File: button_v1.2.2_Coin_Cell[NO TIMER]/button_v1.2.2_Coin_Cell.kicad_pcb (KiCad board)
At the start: 2 copper layers, 21 x 47.8 mm, 18 parts, among them J1 Conn_01x05_Female, SW1 SW_Push, SW2 SW_Push, U1 TPS61097A, X1 ESP-12E

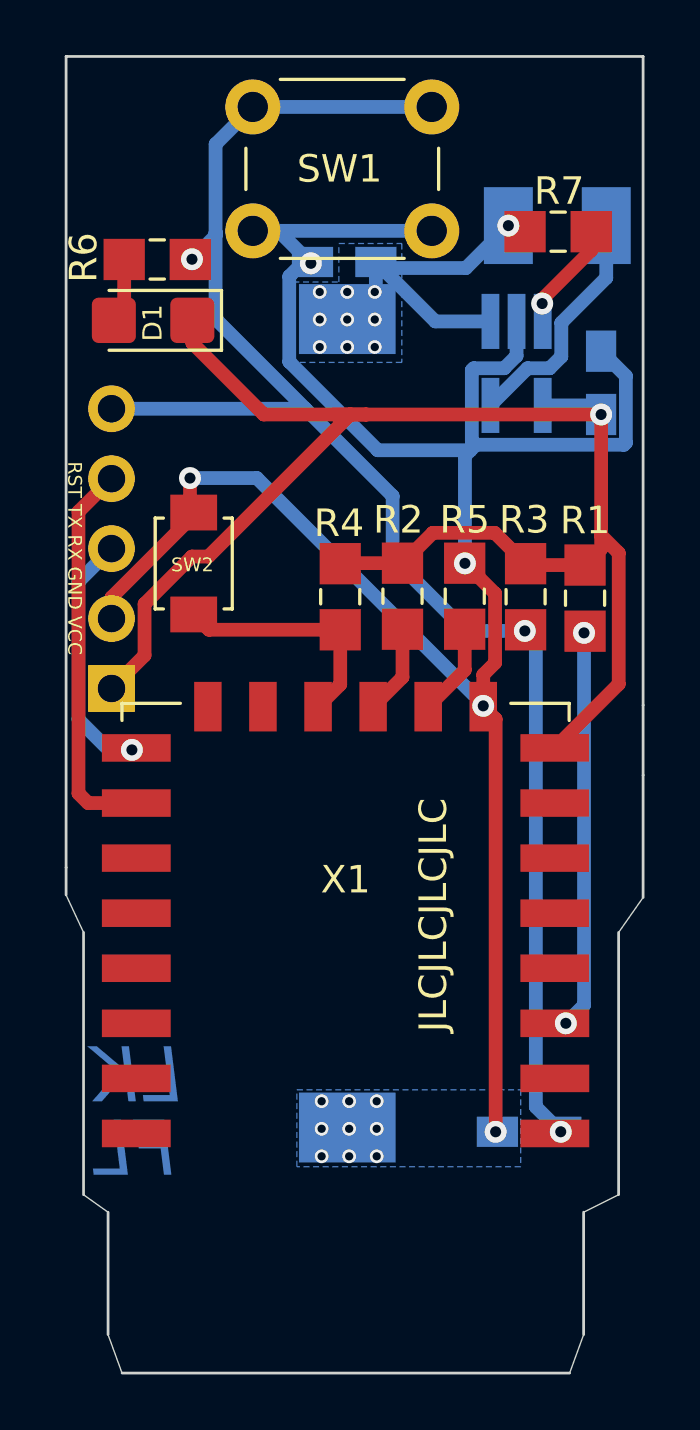
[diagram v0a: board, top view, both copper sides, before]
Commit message: Silkscreen Update
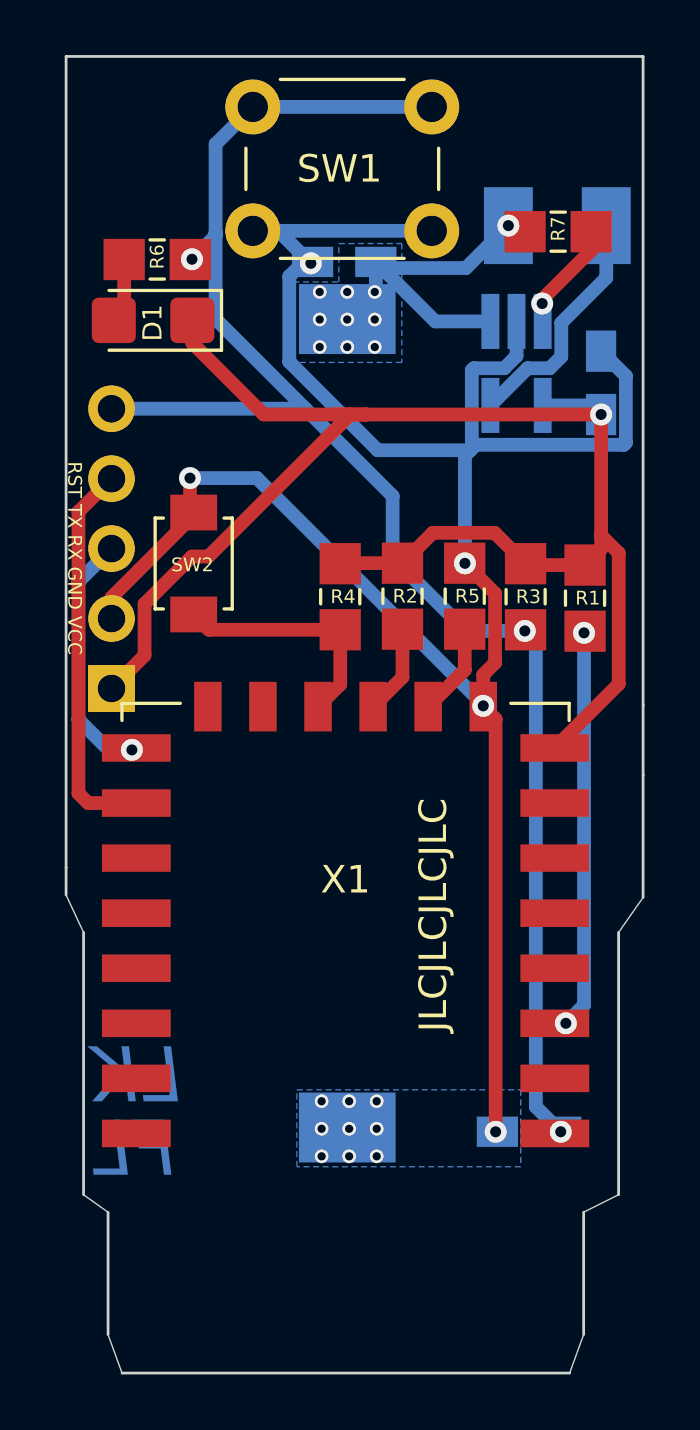
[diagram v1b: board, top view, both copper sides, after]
